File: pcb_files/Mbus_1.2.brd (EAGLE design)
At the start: 101.6 x 71.1 mm, 50 parts, among them IC1 NCP1117ST50T3G, IC3 ATMEGA2560-16AU, IC4 RTC_PCF8523T, J1 F-1X18-SIP-100-32Y, J2 USB_A_SMT_FEMALE, Q1 BSS138, Q2 32.768, Q3 BSS138, T1 2N3904, Y1 CSTCE16M0V53-R0 16MHZ

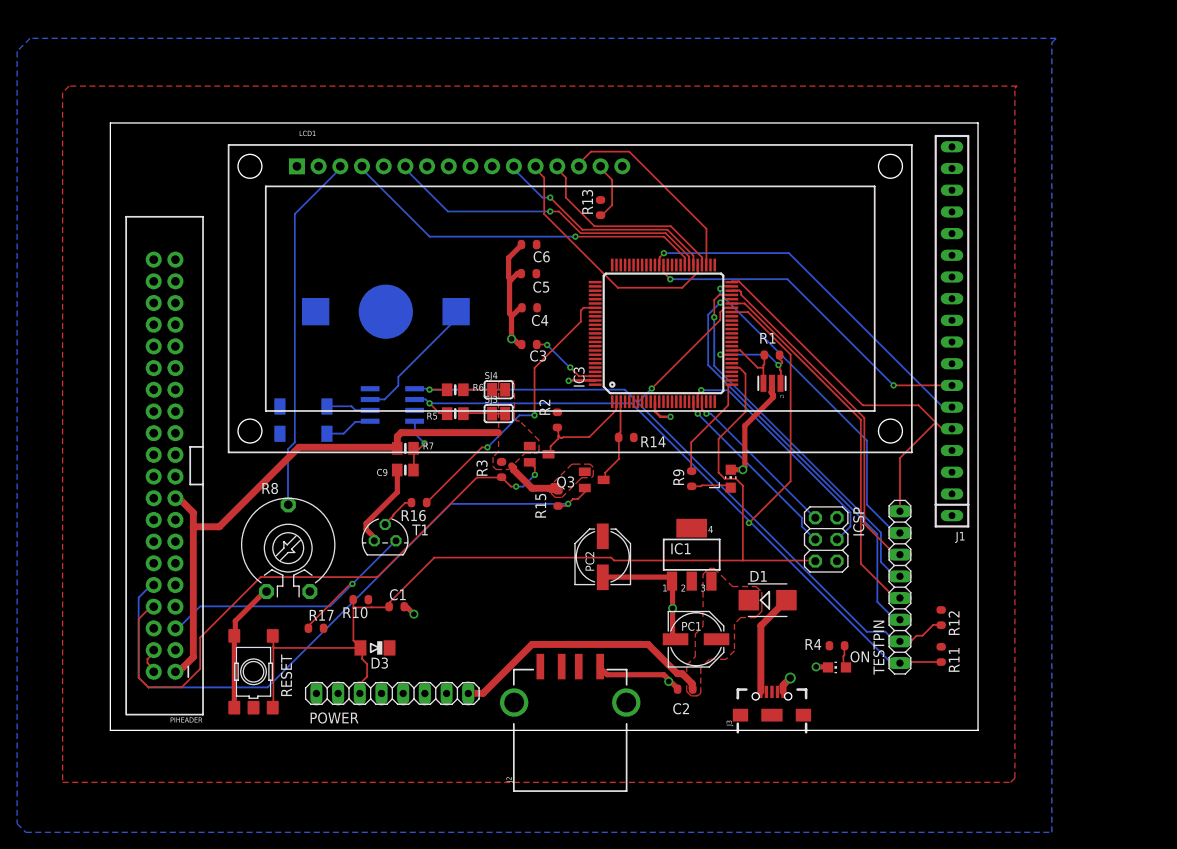
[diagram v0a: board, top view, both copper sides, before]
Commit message: Create gerber files
Signed-off-by: Yiteng Cai <alonsochate@umich.edu>
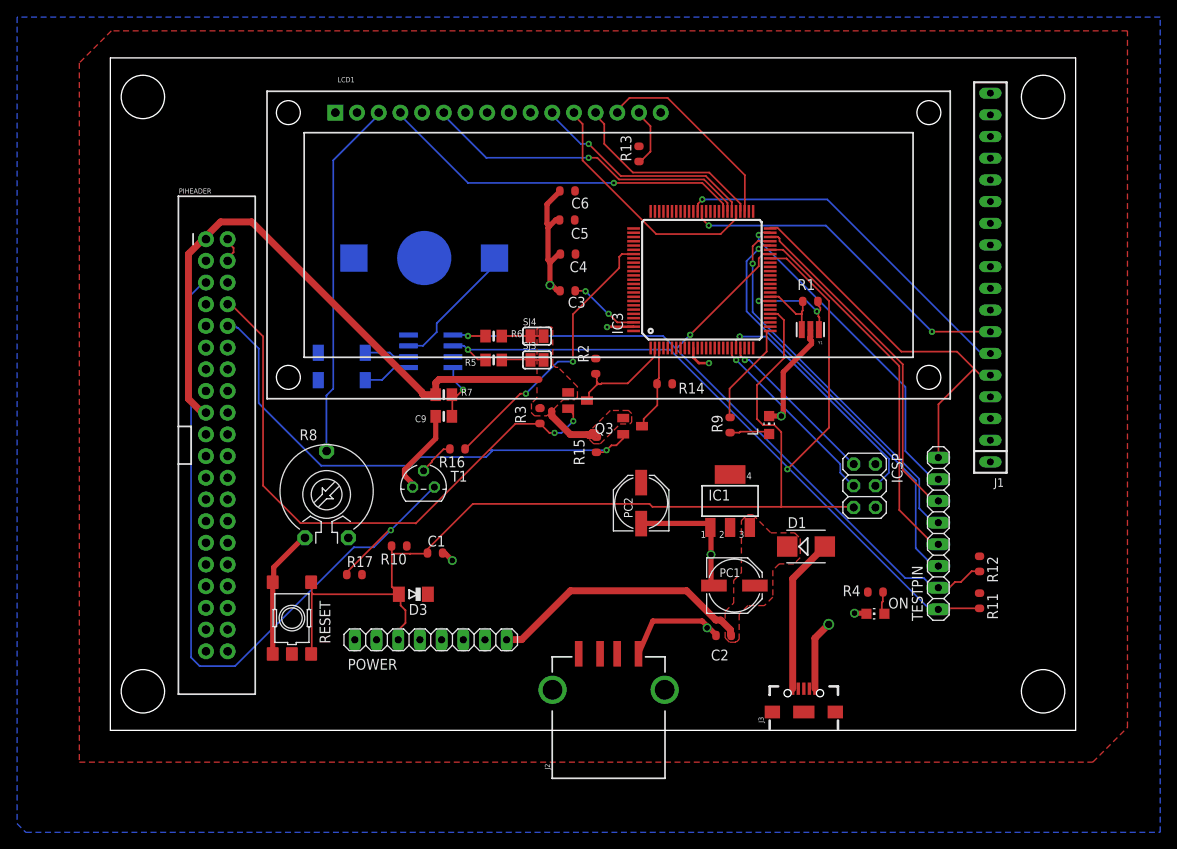
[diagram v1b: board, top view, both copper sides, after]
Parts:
- moved C5 7.73 mm to (53.5, 59.8)
- moved IC3 7.73 mm to (69.3, 52.8)
- moved LCD1 7.73 mm to (58.3, 56.8)
- moved Q1 7.73 mm to (54.7, 38.6)
- moved R9 7.73 mm to (72.6, 35.8)
- moved C1 7.73 mm to (38.0, 20.8)
- moved C2 7.73 mm to (71.8, 11.1)
- moved C9 7.73 mm to (39.0, 36.8)
- moved D3 7.73 mm to (35.5, 15.9)
- moved ICSP 7.73 mm to (88.3, 28.6)
- moved ON 7.73 mm to (89.6, 13.7)
- moved PC1 7.73 mm to (73.1, 17.0)
- moved R11 7.73 mm to (101.8, 15.2)
- moved R15 7.73 mm to (56.9, 33.4)
- moved R17 7.73 mm to (28.6, 18.2)
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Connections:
- removed net RXD2: IC3.12
- removed net TXD2: IC3.13
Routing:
- net OUT: track 37.5 -> 89.9 mm
- net N$12: track 75.7 -> 60.3 mm
- net +3V3: track 71.3 -> 80.5 mm
- net GND: track 92.4 -> 100.6 mm
- net PWRIN: track 12.0 -> 18.2 mm
- net N$5: track 71.3 -> 69.1 mm
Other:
- board size 101.6 x 71.1 mm -> 113 x 78.7 mm
